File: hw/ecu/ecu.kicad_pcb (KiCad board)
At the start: 2 copper layers, 143.8 x 80 mm, 265 parts, among them J1 POWER, J10 CUR_LOOP_IN, J11 SENSORS, J12 VALVE_REG, J13 OUTPUTS, J14 VALVES_FRONT, J15 VALVES_BACK, J2 UART_DEBUG, J3 DEBUG, J4 EXPANSION, J5 SWD, J6 CAN, J7 USB_B_Micro, J8 BUTTONS, J9 ENGINE, Q1 IPD30N06S4L23, Q10 IPD30N06S4L23, Q11 IPD30N06S4L23, Q12 IPD30N06S4L23, Q13 IPD30N06S4L23, Q2 IPD30N06S4L23, Q3 DMP2035, Q4 IPD30N06S4L23, Q5 IPD30N06S4L23, Q6 IPD30N06S4L23, Q7 IPD30N06S4L23, Q8 IPD30N06S4L23, Q9 IPD30N06S4L23, SW1 RESET, U1 M24C64, U2 STM32F072RBTx, U3 TS1117BCW33, U4 MCP2562-E-SN, U5 USB6B1, U6 74HC4050, U7 74HC4050, U8 TSV912

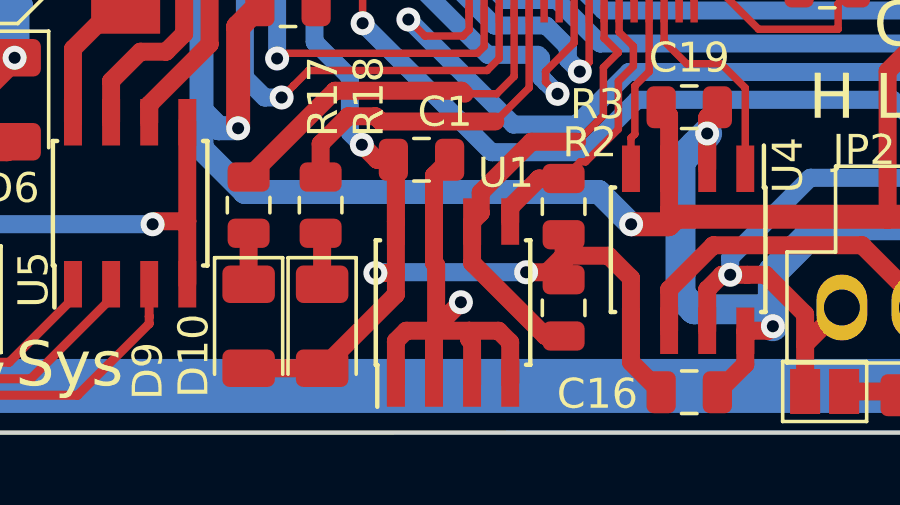
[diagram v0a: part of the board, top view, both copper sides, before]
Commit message: Generated gerbers for ECU
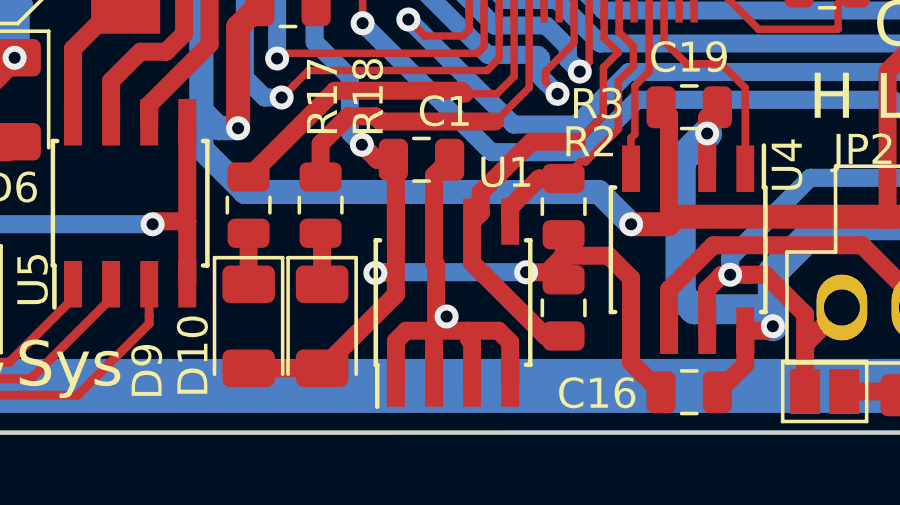
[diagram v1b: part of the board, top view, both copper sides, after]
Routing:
- net GND: track 664.5 -> 663.8 mm
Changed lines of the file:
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@@
-(kicad_pcb (version 20171130) (host pcbnew 5.0.0)
+(kicad_pcb (version 20171130) (host pcbnew 5.0.1)
   (general
     (thickness 1.6)
@@
     (pad_drill 0.762)
     (pad_to_mask_clearance 0.2)
+    (solder_mask_min_width 0.25)
     (aux_axis_origin 0 0)
     (grid_origin 156.375 57.275)
-    (visible_elements FFFDFF7F)
+    (visible_elements FFFDF77F)
     (pcbplotparams
-      (layerselection 0x010fc_ffffffff)
-      (usegerberextensions false)
+      (layerselection 0x010ec_ffffffff)
+      (usegerberextensions true)
       (usegerberattributes false)
       (usegerberadvancedattributes false)
@@
       (psa4output false)
       (plotreference true)
-      (plotvalue true)
+      (plotvalue false)
       (plotinvisibletext false)
       (padsonsilk false)
@@
       (outputformat 1)
       (mirror false)
-      (drillshape 1)
+      (drillshape 0)
       (scaleselection 1)
-      (outputdirectory ""))
+      (outputdirectory "gerber"))
   )
   (net 0 "")
@@
     (tags capacitor)
     (attr smd)
-    (fp_text reference C3 (at 0 1.65 180) (layer B.SilkS)
+    (fp_text reference C3 (at 0.0125 -1.725 180) (layer B.SilkS)
       (effects (font (size 1 1) (thickness 0.15)) (justify mirror))
     )
@@
     (tags capacitor)
     (attr smd)
-    (fp_text reference C4 (at 0 1.65) (layer B.SilkS)
+    (fp_text reference C4 (at -2.8875 0.1) (layer B.SilkS)
       (effects (font (size 1 1) (thickness 0.15)) (justify mirror))
     )
@@
     (tags capacitor)
     (attr smd)
-    (fp_text reference C6 (at 0 1.65) (layer B.SilkS)
+    (fp_text reference C6 (at -2.8375 0.05) (layer B.SilkS)
       (effects (font (size 1 1) (thickness 0.15)) (justify mirror))
     )
@@
     (tags capacitor)
     (attr smd)
-    (fp_text reference C7 (at 0 1.65) (layer B.SilkS)
+    (fp_text reference C7 (at -2.8875 0.025) (layer B.SilkS)
       (effects (font (size 1 1) (thickness 0.15)) (justify mirror))
     )
@@
     (tags capacitor)
     (attr smd)
-    (fp_text reference C9 (at 0 1.65 270) (layer B.SilkS)
+    (fp_text reference C9 (at -0.15 2.25 270) (layer B.SilkS)
       (effects (font (size 1 1) (thickness 0.15)) (justify mirror))
     )
@@
     (tags capacitor)
     (attr smd)
-    (fp_text reference C10 (at 0 1.65) (layer B.SilkS)
+    (fp_text reference C10 (at -3.2875 0.075) (layer B.SilkS)
       (effects (font (size 1 1) (thickness 0.15)) (justify mirror))
     )
@@
     (tags capacitor)
     (attr smd)
-    (fp_text reference C12 (at 0 1.65 270) (layer B.SilkS)
+    (fp_text reference C12 (at -0.1125 -2 270) (layer B.SilkS)
       (effects (font (size 1 1) (thickness 0.15)) (justify mirror))
     )
@@
   (segment (start 170.075 48.32) (end 170.075 49.425) (width 0.6) (layer F.Cu) (net 2))
   (segment (start 170.075 48.32) (end 171.19 48.32) (width 0.7) (layer F.Cu) (net 2))
-  (via (at 145.475 94.1) (size 0.8) (drill 0.4) (layers F.Cu B.Cu) (net 2))
-  (segment (start 144.65 95.05) (end 144.65 94.925) (width 0.6) (layer F.Cu) (net 2))
-  (segment (start 144.65 94.925) (end 145.475 94.1) (width 0.6) (layer F.Cu) (net 2))
   (segment (start 169.825 80.5) (end 169.825 79.775) (width 0.6) (layer F.Cu) (net 2))
   (segment (start 170.62 79.275) (end 171.995 79.275) (width 0.6) (layer F.Cu) (net 2))
@@
   (via (at 100.025 53.415) (size 0.8) (drill 0.4) (layers F.Cu B.Cu) (net 2))
   (segment (start 100.175 52.27) (end 100.025 53.415) (width 1.5) (layer F.Cu) (net 2))
+  (segment (start 144.65 94.925) (end 144.65 95.05) (width 0.6) (layer F.Cu) (net 2))
+  (via (at 145 94.575) (size 0.8) (drill 0.4) (layers F.Cu B.Cu) (net 2))
+  (segment (start 145 94.575) (end 144.65 94.925) (width 0.6) (layer F.Cu) (net 2))
   (segment (start 156.75 83.575) (end 154.7 83.575) (width 0.25) (layer F.Cu) (net 3))
   (segment (start 154.7 83.575) (end 154 82.875) (width 0.25) (layer F.Cu) (net 3))

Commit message: Updated few resistors/capacitors values on board
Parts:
- C20, C21: value 100n -> 1u
- C32, C33, C34, C35, C36, C37: value 100n -> 680n
- R13: value 91k -> 22k
- R14: value 13k -> 3k3
- R15: value 36k -> 33k
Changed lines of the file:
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@@
     (aux_axis_origin 0 0)
     (grid_origin 156.375 57.275)
-    (visible_elements FFFDF77F)
+    (visible_elements FFFBF77F)
     (pcbplotparams
       (layerselection 0x010ec_ffffffff)
@@
       (effects (font (size 1 1) (thickness 0.15)))
     )
-    (fp_text value 100n (at 0 1.65 180) (layer F.Fab)
+    (fp_text value 1u (at 0 1.65 180) (layer F.Fab)
       (effects (font (size 1 1) (thickness 0.15)))
     )
@@
       (effects (font (size 1 1) (thickness 0.15)))
     )
-    (fp_text value 100n (at 0 1.65) (layer F.Fab)
+    (fp_text value 1u (at 0 1.65) (layer F.Fab)
       (effects (font (size 1 1) (thickness 0.15)))
     )
@@
       (effects (font (size 1 1) (thickness 0.15)))
     )
-    (fp_text value 100n (at 0 1.65 90) (layer F.Fab)
+    (fp_text value 680n (at 0 1.65 90) (layer F.Fab)
       (effects (font (size 1 1) (thickness 0.15)))
     )
@@
       (effects (font (size 1 1) (thickness 0.15)))
     )
-    (fp_text value 100n (at 0 1.65 90) (layer F.Fab)
+    (fp_text value 680n (at 0 1.65 90) (layer F.Fab)
       (effects (font (size 1 1) (thickness 0.15)))
     )
@@
       (effects (font (size 1 1) (thickness 0.15)))
     )
-    (fp_text value 100n (at 0 1.65 90) (layer F.Fab)
+    (fp_text value 680n (at 0 1.65 90) (layer F.Fab)
       (effects (font (size 1 1) (thickness 0.15)))
     )
@@
       (effects (font (size 1 1) (thickness 0.15)))
     )
-    (fp_text value 100n (at 0 1.65 90) (layer F.Fab)
+    (fp_text value 680n (at 0 1.65 90) (layer F.Fab)
       (effects (font (size 1 1) (thickness 0.15)))
     )
@@
       (effects (font (size 1 1) (thickness 0.15)))
     )
-    (fp_text value 100n (at 0 1.65 90) (layer F.Fab)
+    (fp_text value 680n (at 0 1.65 90) (layer F.Fab)
       (effects (font (size 1 1) (thickness 0.15)))
     )
@@
       (effects (font (size 1 1) (thickness 0.15)))
     )
-    (fp_text value 100n (at 0 1.65 90) (layer F.Fab)
+    (fp_text value 680n (at 0 1.65 90) (layer F.Fab)
       (effects (font (size 1 1) (thickness 0.15)))
     )
@@
       (effects (font (size 1 1) (thickness 0.15)))
     )
-    (fp_text value 91k (at 0 1.65) (layer F.Fab)
+    (fp_text value 22k (at 0 1.65) (layer F.Fab)
       (effects (font (size 1 1) (thickness 0.15)))
     )
@@
       (effects (font (size 1 1) (thickness 0.15)))
     )
-    (fp_text value 13k (at 0 1.65 180) (layer F.Fab)
+    (fp_text value 3k3 (at 0 1.65 180) (layer F.Fab)
       (effects (font (size 1 1) (thickness 0.15)))
     )
@@
       (effects (font (size 1 1) (thickness 0.15)))
     )
-    (fp_text value 36k (at 0 1.65 180) (layer F.Fab)
+    (fp_text value 33k (at 0 1.65 180) (layer F.Fab)
       (effects (font (size 1 1) (thickness 0.15)))
     )

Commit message: Updated schematic to latest changes in usb protection ic
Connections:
- J7 pad 1: Net-(J7-Pad1) -> Net-(D7-Pad2)
- U5 pad 1: Net-(J7-Pad1) -> Net-(D7-Pad2)
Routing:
- net Net-(D7-Pad2): track 4.93 -> 12.4 mm
- net Net-(J7-Pad1): track 7.46 -> 0.00 mm
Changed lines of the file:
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@@
     (zones 0)
     (modules 265)
-    (nets 170)
+    (nets 169)
   )
   (page A4)
@@
   (net 167 "Net-(J4-Pad4)")
   (net 168 "Net-(C46-Pad2)")
-  (net 169 "Net-(J7-Pad1)")
   (net_class Default "Toto je výchozí třída sítě."
     (clearance 0.25)
@@
     (add_net "Net-(J4-Pad3)")
     (add_net "Net-(J4-Pad4)")
-    (add_net "Net-(J7-Pad1)")
     (add_net "Net-(J7-Pad2)")
     (add_net "Net-(J7-Pad3)")
@@
       (net 2 GND))
     (pad 1 smd rect (at -1.3 -0.825 180) (size 0.45 1.5) (layers F.Cu F.Paste F.Mask)
-      (net 169 "Net-(J7-Pad1)"))
+      (net 24 "Net-(D7-Pad2)"))
     (pad 6 thru_hole oval (at -2.8 -1.075 180) (size 1.8 1.1) (drill oval 1.2 0.5) (layers *.Cu *.Mask)
       (net 2 GND))
@@
     (fp_line (start -2.075 -2.525) (end -3.475 -2.525) (layer F.SilkS) (width 0.15))
     (pad 1 smd rect (at -2.7 -1.905 90) (size 1.55 0.6) (layers F.Cu F.Paste F.Mask)
-      (net 169 "Net-(J7-Pad1)"))
+      (net 24 "Net-(D7-Pad2)"))
     (pad 2 smd rect (at -2.7 -0.635 90) (size 1.55 0.6) (layers F.Cu F.Paste F.Mask)
       (net 89 "Net-(J7-Pad2)"))
@@
   (segment (start 199.725 80.825) (end 199.075 81.475) (width 1) (layer F.Cu) (net 168))
   (segment (start 199.075 81.475) (end 198.775 81.775) (width 1) (layer F.Cu) (net 168))
-  (segment (start 127.3 94.775) (end 127.3 95.3) (width 0.3) (layer F.Cu) (net 169))
-  (segment (start 128.099978 96.099978) (end 130.420022 96.099978) (width 0.3) (layer F.Cu) (net 169))
-  (segment (start 132.545 93.975) (end 132.545 93.5) (width 0.3) (layer F.Cu) (net 169))
-  (segment (start 127.3 95.3) (end 128.099978 96.099978) (width 0.3) (layer F.Cu) (net 169))
-  (segment (start 130.420022 96.099978) (end 132.545 93.975) (width 0.3) (layer F.Cu) (net 169))
+  (segment (start 127.3 94.775) (end 127.3 95.3) (width 0.3) (layer F.Cu) (net 24))
+  (segment (start 128.099978 96.099978) (end 130.420022 96.099978) (width 0.3) (layer F.Cu) (net 24))
+  (segment (start 132.545 93.975) (end 132.545 93.5) (width 0.3) (layer F.Cu) (net 24))
+  (segment (start 127.3 95.3) (end 128.099978 96.099978) (width 0.3) (layer F.Cu) (net 24))
+  (segment (start 130.420022 96.099978) (end 132.545 93.975) (width 0.3) (layer F.Cu) (net 24))
   (zone (net 2) (net_name GND) (layer B.Cu) (hatch edge 0.508)
     (connect_pads (clearance 0.5))
